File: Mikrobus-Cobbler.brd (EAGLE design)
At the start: 54.6 x 36.8 mm, 2 parts

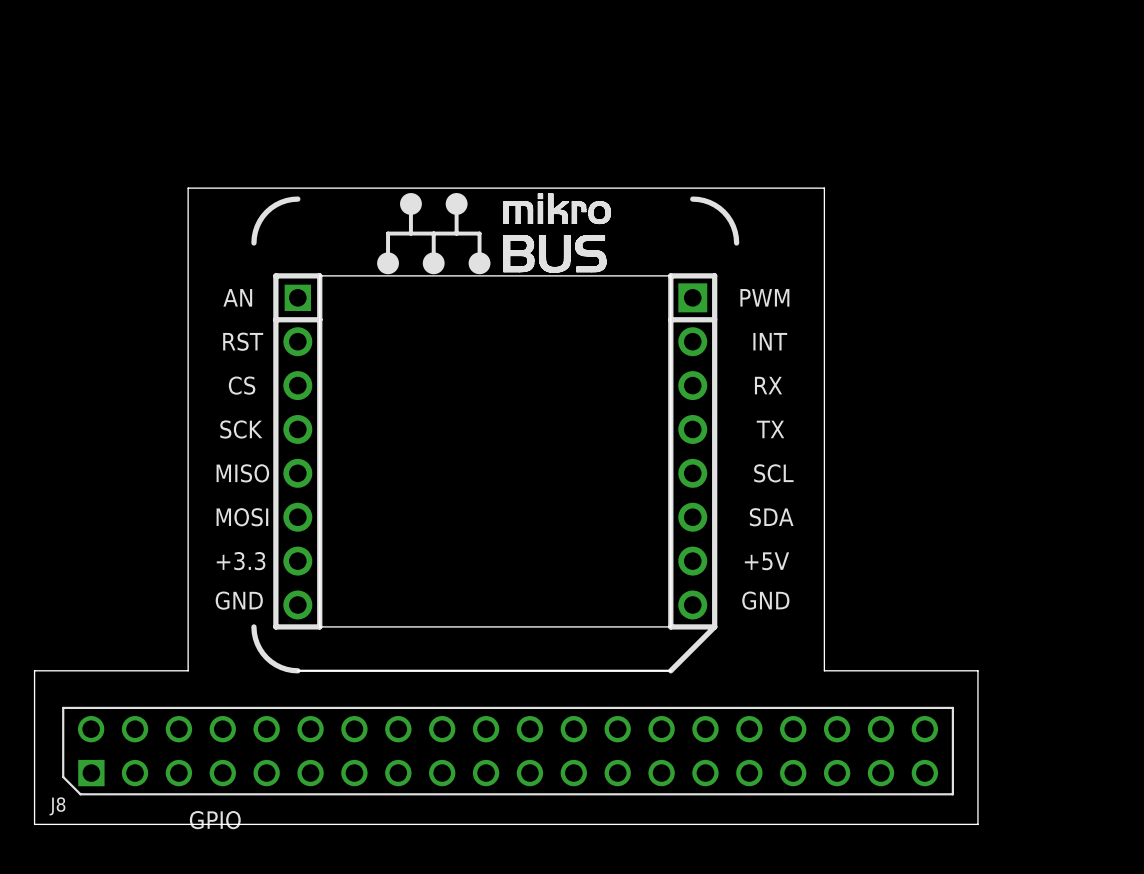
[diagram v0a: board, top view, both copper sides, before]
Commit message: Adjusted and Routed PCB
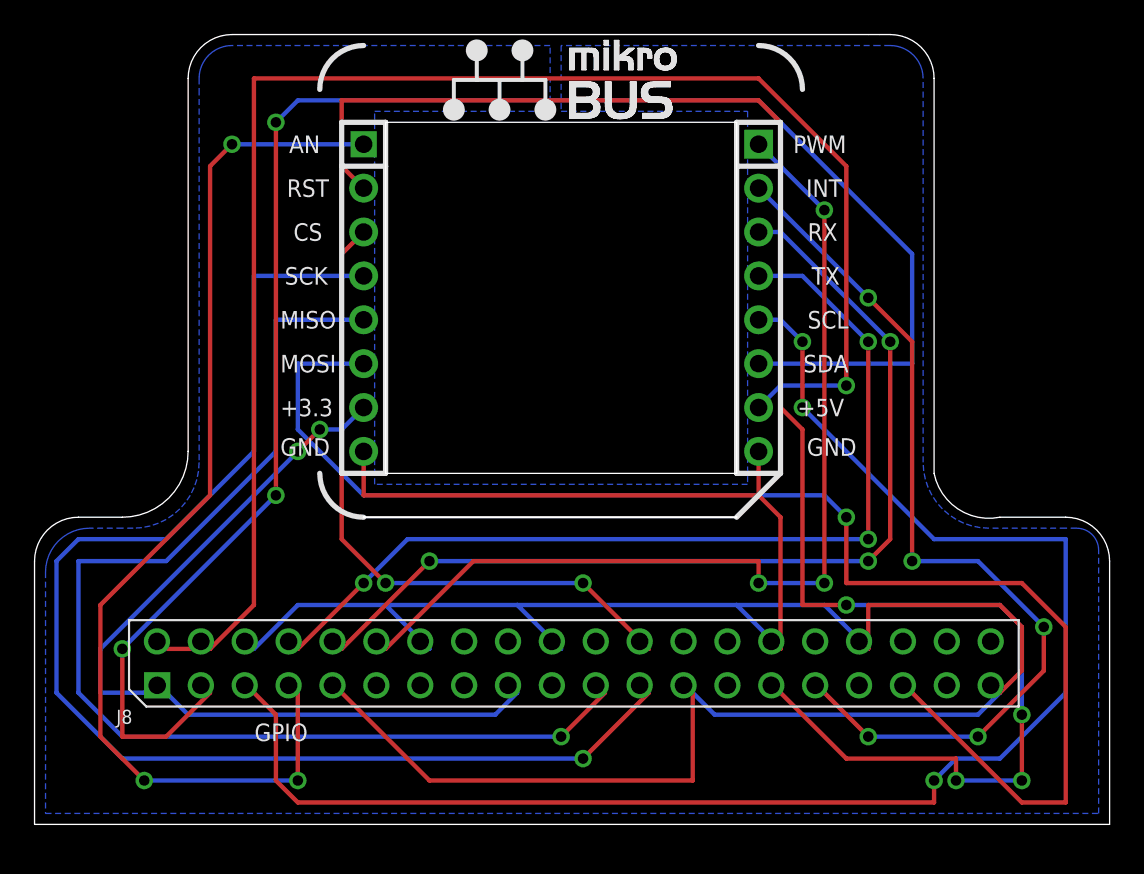
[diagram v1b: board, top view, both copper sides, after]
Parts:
- moved MB1 9.67 mm to (30.5, 31.8)
- moved PCB1 6.35 mm to (0.00, 3.81)
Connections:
- net N$1 renamed GND
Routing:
- net GND: track 0.00 -> 156.7 mm
- net N$15: track 0.00 -> 102.3 mm, vias 0 -> 3
- net N$5: track 0.00 -> 99.6 mm, vias 0 -> 4
- net N$2: track 0.00 -> 92.7 mm, vias 0 -> 1
- net N$14: track 0.00 -> 90.1 mm, vias 0 -> 3
- net N$9: track 0.00 -> 81.4 mm, vias 0 -> 1
- net N$6: track 0.00 -> 76.3 mm, vias 0 -> 1
- net N$8: track 0.00 -> 67.7 mm, vias 0 -> 1
- net N$4: track 0.00 -> 63.3 mm, vias 0 -> 3
- net N$12: track 0.00 -> 56.7 mm, vias 0 -> 3
- net N$10: track 0.00 -> 56.4 mm, vias 0 -> 3
- net N$13: track 0.00 -> 55.7 mm, vias 0 -> 3
- net N$11: track 0.00 -> 53.0 mm, vias 0 -> 5
- net N$3: track 0.00 -> 49.7 mm, vias 0 -> 2
- net N$7: track 0.00 -> 39.4 mm, vias 0 -> 2
- added copper zone on layer 16, net GND
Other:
- board size 54.6 x 36.8 mm -> 62.2 x 45.7 mm
